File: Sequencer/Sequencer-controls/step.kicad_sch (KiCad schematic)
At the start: 5 parts, among them SW18 SW_SPDT

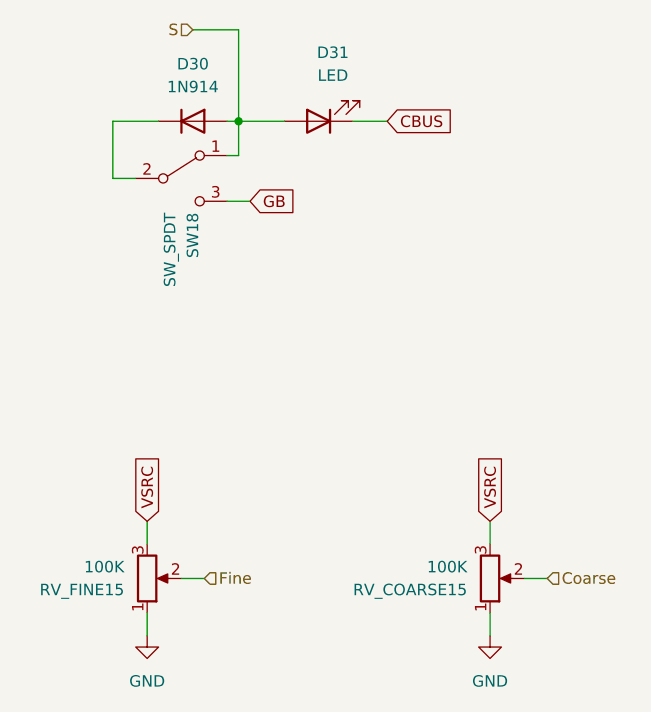
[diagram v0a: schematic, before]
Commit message: misc
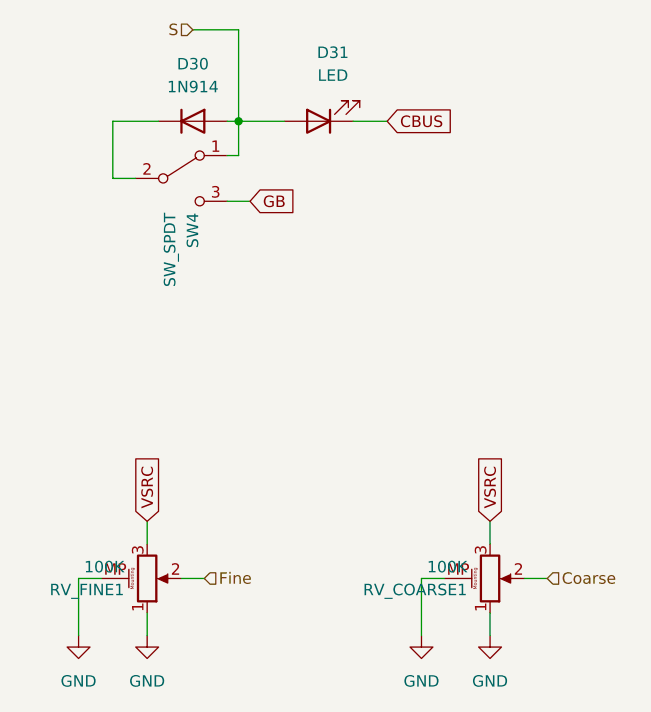
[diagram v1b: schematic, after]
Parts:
- RV_COARSE1: renamed from RV_COARSE15; symbol Device:R_Potentiometer -> Device:R_Potentiometer_MountingPin
- RV_FINE1: renamed from RV_FINE15; symbol Device:R_Potentiometer -> Device:R_Potentiometer_MountingPin
- renumbered SW18 to SW4
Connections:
- net GND: now also RV_COARSE1.MP (MountPin), RV_FINE1.MP (MountPin)
